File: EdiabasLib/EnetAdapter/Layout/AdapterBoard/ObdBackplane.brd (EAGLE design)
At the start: 36 x 20 mm, 11 parts, among them J1 OBDII, U1 FPC-FFC-CONNECTOR-08-1MM, U2 FPC-FFC-CONNECTOR-08-1MM-L

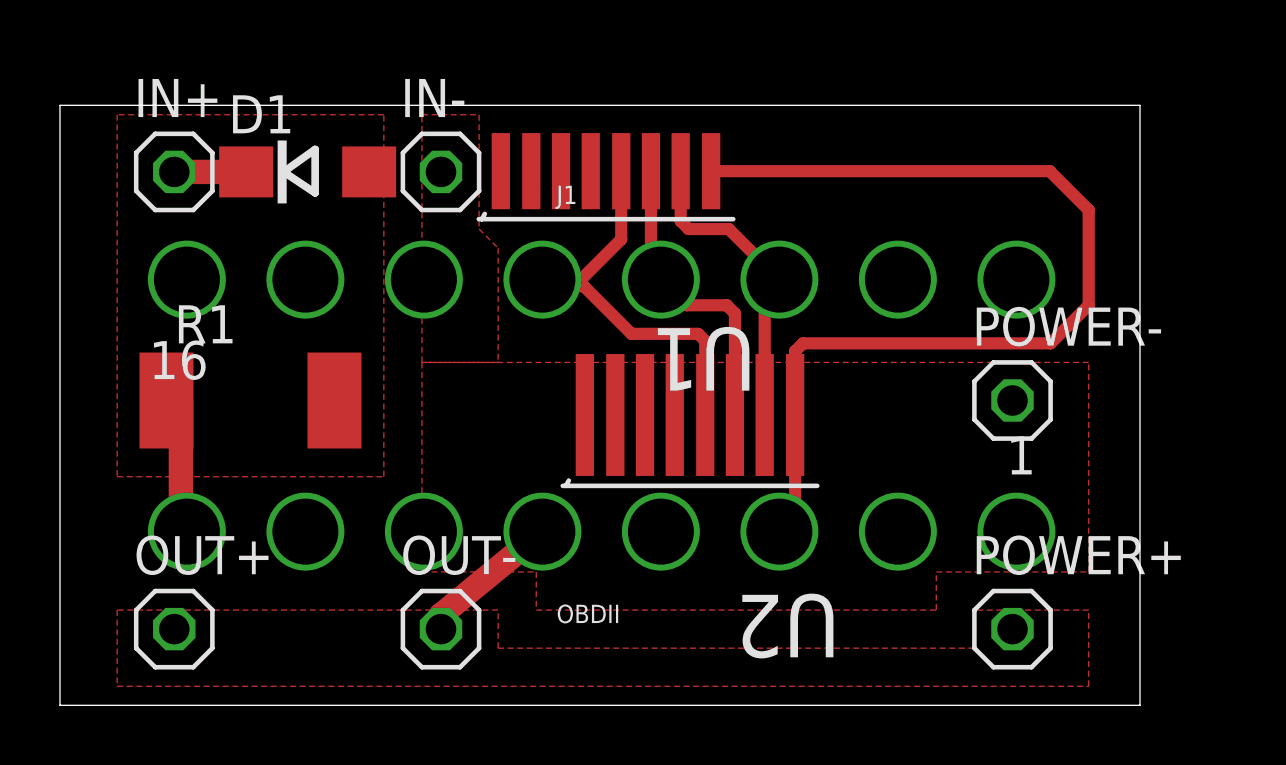
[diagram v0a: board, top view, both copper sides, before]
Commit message: Layout for elecrow
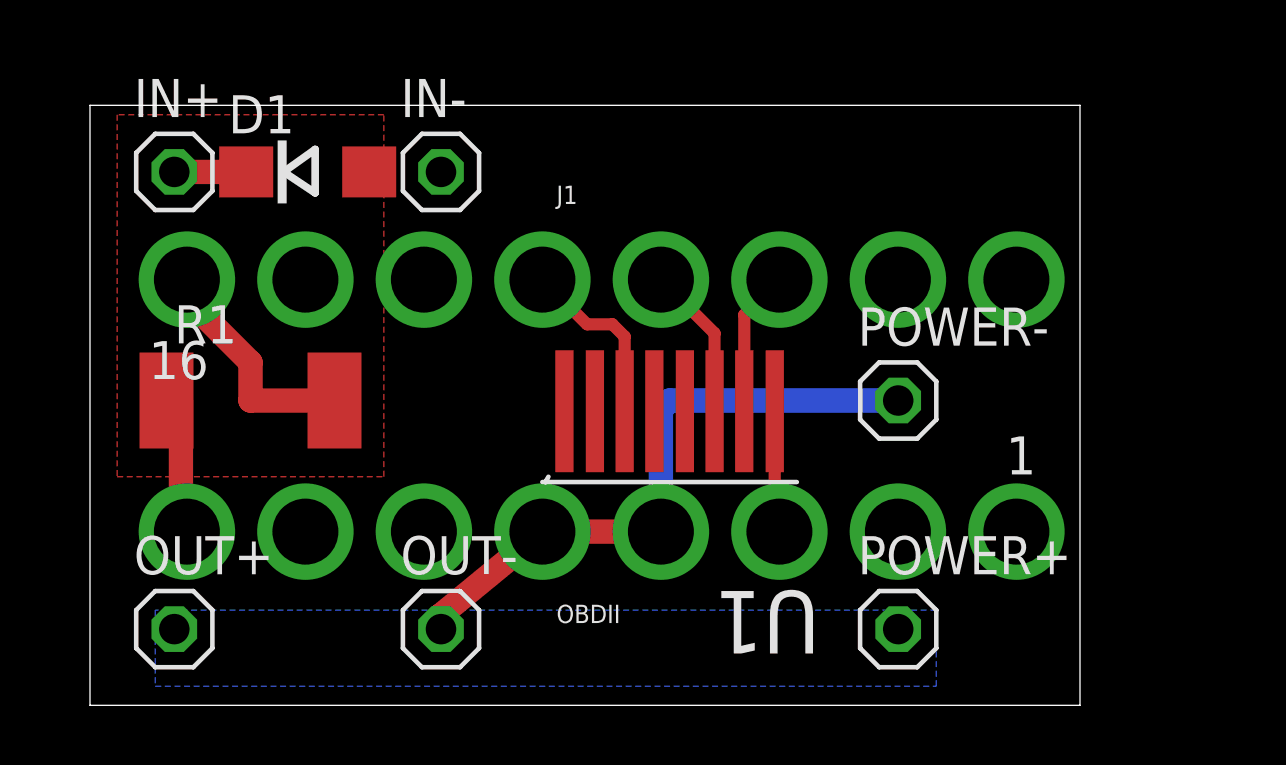
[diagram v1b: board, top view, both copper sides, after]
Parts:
- removed U2: FPC-FFC-CONNECTOR-08-1MM-L, obd_special:FPC-FFC-CONNECTOR-08-1MM-L
- U1: value FPC-FFC-CONNECTOR-08-1MM -> FPC-FFC-CONNECTOR-08-1MM-L; device obd_special:FPC-FFC-CONNECTOR-08-1MM -> obd_special:FPC-FFC-CONNECTOR-08-1MM-L
- moved U1 9.02 mm to (20.3, 7.75)
- moved POWER+ 3.81 mm to (27.9, 2.54)
- moved POWER- 3.81 mm to (27.9, 10.2)
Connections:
- net GND: no longer IN-.1
- net N$3: no longer U2.8
- net N$4: no longer U2.7
- net N$5: no longer U2.6
- net N$6: now also U1.3; no longer U1.5, U2.5
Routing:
- net N$3: track 32.9 -> 4.08 mm
- net GND: track 4.85 -> 20.9 mm
- net +12V: track 0.00 -> 7.71 mm
- net N$6: track 13.2 -> 6.02 mm
- net N$4: track 10.5 -> 4.87 mm
- net N$5: track 10.1 -> 5.13 mm
- added copper zone on layer 16, net +5V
- removed copper zone on layer 1, net +5V
- removed copper zone on layer 1, net GND
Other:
- board size 36 x 20 mm -> 33 x 20 mm
